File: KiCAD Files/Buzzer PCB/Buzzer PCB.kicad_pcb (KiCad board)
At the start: 2 copper layers, 25.2 x 22.9 mm, 13 parts, among them J1 JST-PH Battery IN, J2 JST-PH Feather BAT OUT, J4 Feather D13, Q1 S8050, SW1 SS12D00G5

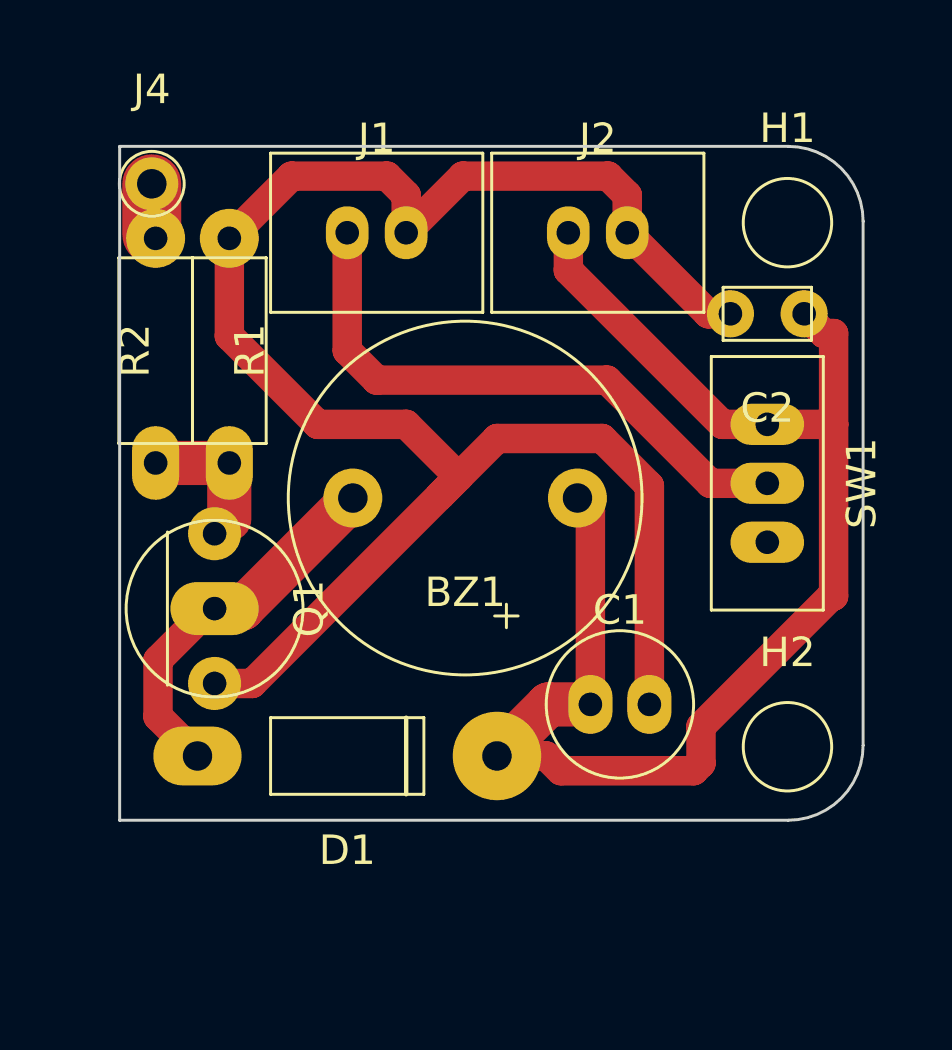
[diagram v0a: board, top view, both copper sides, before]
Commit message: V2 PCB done
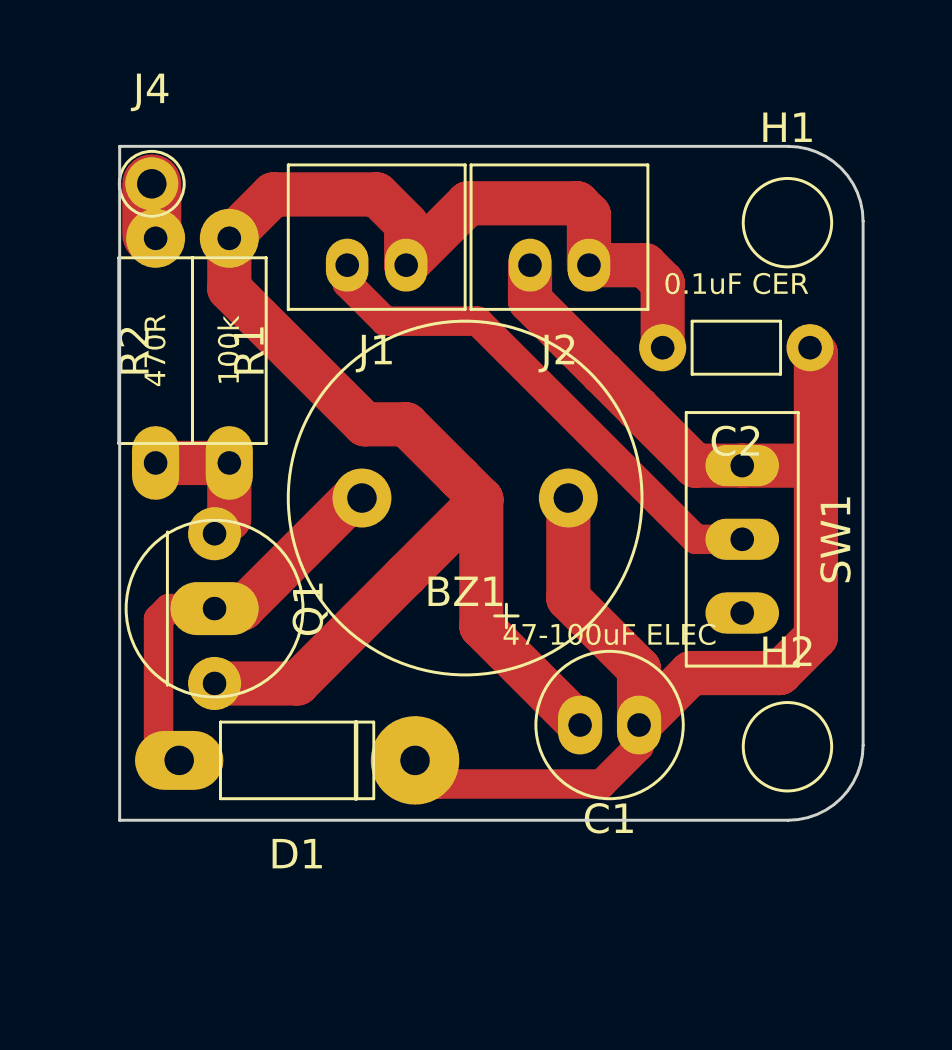
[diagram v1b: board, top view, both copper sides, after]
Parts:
- C1: value 47-100uF -> 47-100uF ELEC
- C2: value 0.1uF -> 0.1uF CER
- J1, J2: footprint Connector_JST:JST_PH_S2B-PH-K_1x02_P2.00mm_Horizontal -> Connector_JST:JST_PH_B2B-PH-K_1x02_P2.00mm_Vertical
- moved SW1 2.08 mm to (105.9, 104.9)
- moved D1 1.71 mm to (90.8, 112.4)
- moved C2 1.56 mm to (105.7, 98.4)
- moved J1 1.49 mm to (94.5, 95.6), turned to 180 degrees
- moved J2 1.14 mm to (100.7, 95.6), turned to 180 degrees
- moved C1 0.78 mm to (101.4, 111.2), turned to 180 degrees
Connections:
- J1 pad 1: BAT_IN -> GND
- J1 pad 2: GND -> BAT_IN
- J2 pad 1: SW_BAT -> GND
- J2 pad 2: GND -> SW_BAT
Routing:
- net GND: track 63.1 -> 56.5 mm
- net BAT_IN: track 20.1 -> 17.6 mm
- net BUZZER_LOW: track 12.7 -> 13.4 mm

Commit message: two_sided
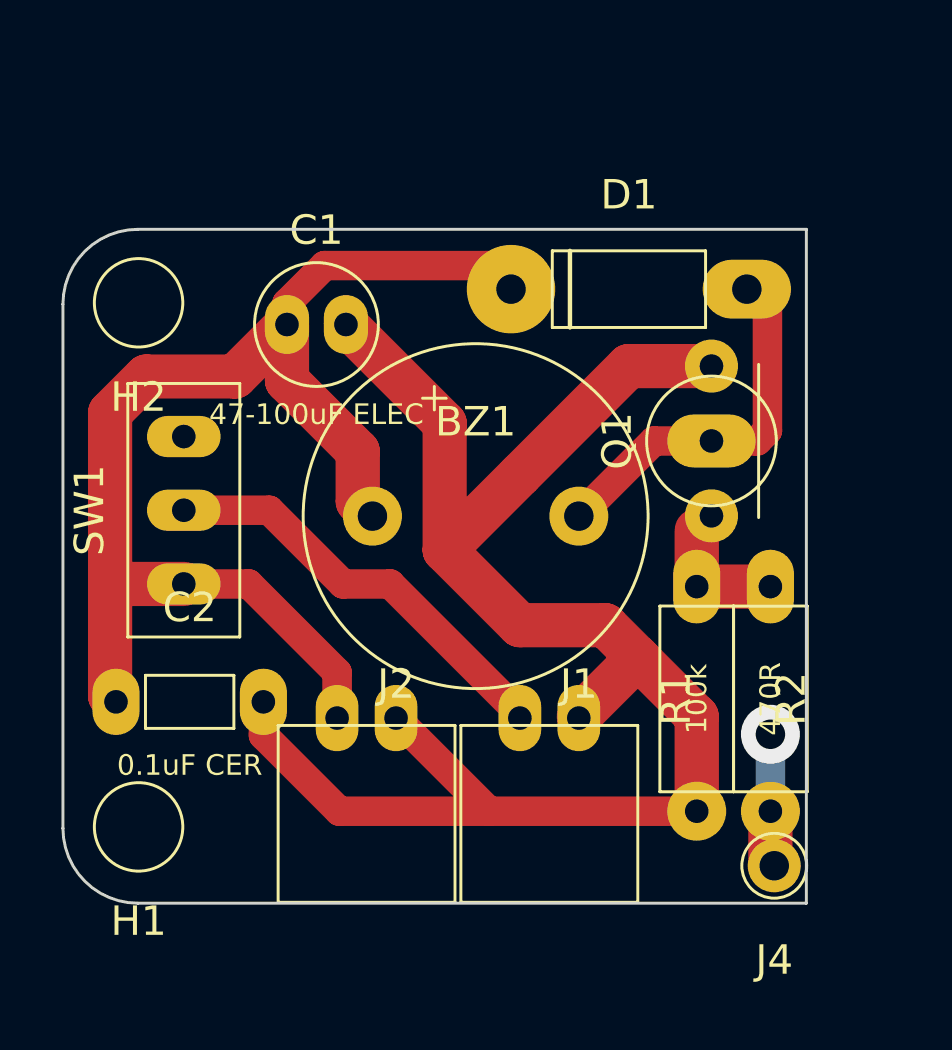
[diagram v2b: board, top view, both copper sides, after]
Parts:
- J1, J2: footprint Connector_JST:JST_PH_B2B-PH-K_1x02_P2.00mm_Vertical -> Connector_JST:JST_PH_S2B-PH-K_1x02_P2.00mm_Horizontal
- moved J4 31.3 mm to (107.0, 116.0), turned to 180 degrees
- moved H1 30.1 mm to (85.4, 114.7), turned to 180 degrees
- moved H2 26.7 mm to (85.4, 96.9), turned to 180 degrees
- moved R1 24.0 mm to (106.9, 110.3), turned to 90 degrees
- moved C2 22.1 mm to (87.2, 110.4), turned to 0 degrees
- moved R2 19.8 mm to (104.4, 110.3), turned to -90 degrees
- moved D1 19.6 mm to (102.1, 96.4), turned to 0 degrees
- moved SW1 19.0 mm to (87.0, 103.9), turned to 90 degrees
- moved J2 18.7 mm to (93.2, 112.7), turned to 0 degrees
- moved J1 17.8 mm to (99.4, 112.7), turned to 0 degrees
- moved Q1 17.8 mm to (104.9, 101.6), turned to 90 degrees
- moved C1 16.8 mm to (91.5, 97.6), turned to 0 degrees
- moved BZ1 0.71 mm to (96.9, 104.1), turned to 0 degrees
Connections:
- J1 pad 1: GND -> BAT_IN
- J1 pad 2: BAT_IN -> GND
- J2 pad 1: GND -> SW_BAT
- J2 pad 2: SW_BAT -> GND
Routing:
- net D13: track 1.90 -> 6.42 mm, vias 0 -> 1
- net SW_BAT: track 48.2 -> 44.5 mm
- net BAT_IN: track 17.6 -> 14.4 mm
- net GND: track 56.5 -> 59.0 mm
- net BUZZER_LOW: track 13.4 -> 12.7 mm
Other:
- outline, holes or cut-outs redrawn
